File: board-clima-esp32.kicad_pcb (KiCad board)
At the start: 2 copper layers, 64.8 x 39.9 mm, 33 parts, among them IC1 ESP32-S3-WROOM-1-N4, J1 Conn_01x02_Pin, J2 Screw_Terminal_01x03, J3 Conn_01x04_Pin, J4 Conn_01x04_Pin, J5 Conn_01x04_Pin, J6 USB_C_Receptacle, Q1 AO3400A, SW1 RESET, SW2 BOOT, U1 AMS1117-3.3, U2 JZC-32F/C

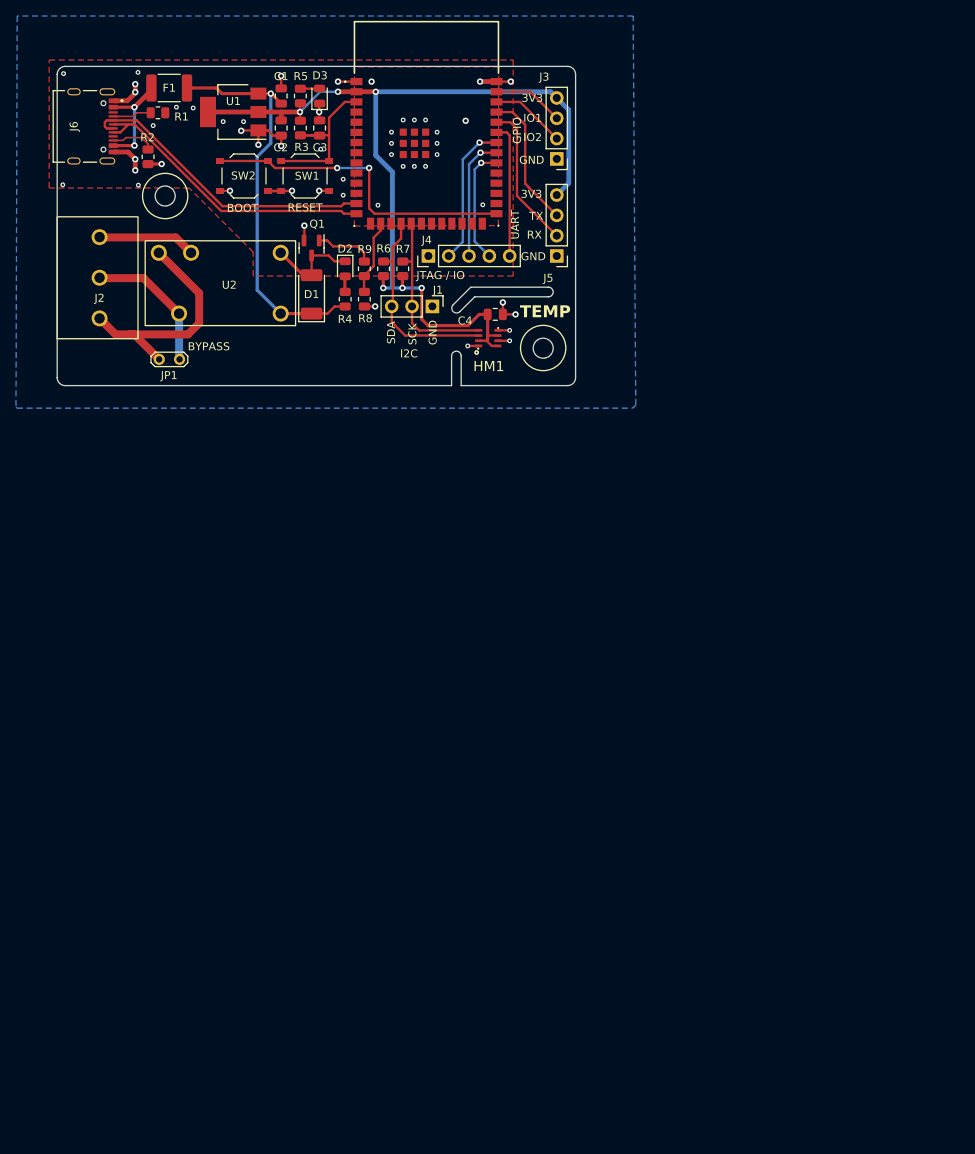
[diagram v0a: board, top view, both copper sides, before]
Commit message: pcb rev2 placement
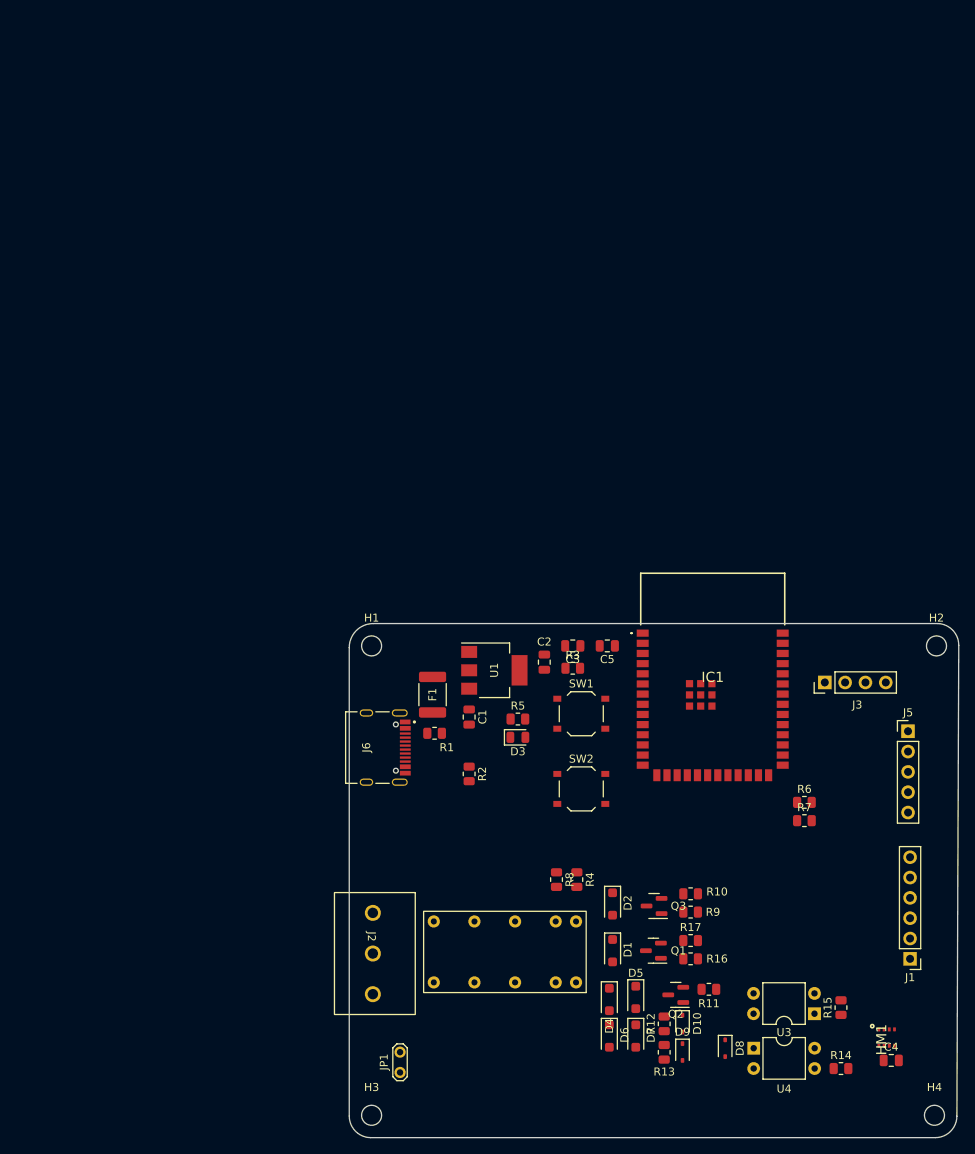
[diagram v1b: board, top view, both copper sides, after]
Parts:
- removed J4: Conn_01x04_Pin, Connector_PinHeader_2.54mm:PinHeader_1x05_P2.54mm_Vertical
- added C5: 1u, Capacitor_SMD:C_0805_2012Metric, F.Cu at (159.8, 126.2)
- added D10: 15V, Diode_SMD:D_SOD-323, F.Cu at (169.2, 173.4)
- added D4: SM4007PL, Diode_SMD:D_SOD-123F, F.Cu at (160.0, 170.4)
- added D5: SM4007PL, Diode_SMD:D_SOD-123F, F.Cu at (163.3, 170.2)
- added D6: SM4007PL, Diode_SMD:D_SOD-123F, F.Cu at (160.0, 175.0)
- added D7: SM4007PL, Diode_SMD:D_SOD-123F, F.Cu at (163.3, 175.0)
- added D8: 4V3, Diode_SMD:D_SOD-323, F.Cu at (174.5, 176.5)
- added D9: 4V7, Diode_SMD:D_SOD-323, F.Cu at (169.2, 177.0)
- added H3: MountingHole, MountingHole:MountingHole_2.5mm, F.Cu at (130.3, 184.9)
- added H4: MountingHole, MountingHole:MountingHole_2.5mm, F.Cu at (200.7, 184.9)
- added Q2: AO3401A, Package_TO_SOT_SMD:SOT-23, F.Cu at (168.3, 169.9)
- added Q3: AO3400A, Package_TO_SOT_SMD:SOT-23, F.Cu at (165.6, 158.8)
- added R10: 10k, Resistor_SMD:R_0805_2012Metric, F.Cu at (170.2, 157.2)
- added R11: 330, Resistor_SMD:R_0805_2012Metric, F.Cu at (172.5, 169.2)
- added R12: 220, Resistor_SMD:R_0805_2012Metric, F.Cu at (166.9, 173.5)
- added R13: 100, Resistor_SMD:R_0805_2012Metric, F.Cu at (166.9, 177.0)
- added R14: 10k, Resistor_SMD:R_0805_2012Metric, F.Cu at (189.0, 179.1)
- added R15: 330, Resistor_SMD:R_0805_2012Metric, F.Cu at (189.0, 171.4)
- added R16: 220, Resistor_SMD:R_0805_2012Metric, F.Cu at (170.2, 165.4)
- added R17: 10k, Resistor_SMD:R_0805_2012Metric, F.Cu at (170.2, 163.1)
- added U3: PC817, Package_DIP:DIP-4_W7.62mm, F.Cu at (185.7, 172.2)
- added U4: PC817, Package_DIP:DIP-4_W7.62mm, F.Cu at (178.1, 176.5)
- D1: value SM4007 -> SM4007PL; footprint Diode_SMD:D_MELF -> Diode_SMD:D_SOD-123F
- D2: value LED -> SM4007PL; footprint LED_SMD:LED_0805_2012Metric -> Diode_SMD:D_SOD-123F
- J1: value Conn_01x02_Pin -> Conn_01x06_Pin; footprint Connector_PinHeader_2.54mm:PinHeader_1x03_P2.54mm_Vertical -> Connector_PinHeader_2.54mm:PinHeader_1x06_P2.54mm_Vertical
- J5: value Conn_01x04_Pin -> Conn_01x05_Pin; footprint Connector_PinHeader_2.54mm:PinHeader_1x04_P2.54mm_Vertical -> Connector_PinHeader_2.54mm:PinHeader_1x05_P2.54mm_Vertical
- R4: value 220 -> 0
- R5: value 220 -> 1k
- R8: value 10k -> 0
- U2: value JZC-32F/C -> ~; footprint JZC-32FC:JZC-32FC -> HFD2:HFD2-00X-M-L2
- moved C4 105.6 mm to (195.3, 178.1)
- moved J1 101.1 mm to (197.6, 165.4), turned to 180 degrees
- moved HM1 99.7 mm to (193.7, 176.2), turned to 90 degrees
- moved Q1 97.7 mm to (165.5, 164.3), turned to 180 degrees
- moved JP1 93.3 mm to (133.9, 179.6), turned to 90 degrees
- moved U2 90.9 mm to (157.1, 169.6)
- moved D1 90.3 mm to (160.4, 164.3), turned to -90 degrees
- moved R9 90.2 mm to (170.2, 159.5), turned to 0 degrees
- moved SW2 87.4 mm to (156.5, 144.1)
- moved R2 87.0 mm to (142.5, 142.2)
- moved D2 86.1 mm to (160.4, 158.5)
- moved J6 85.8 mm to (129.7, 138.9)
- moved R7 85.3 mm to (184.4, 148.1), turned to 0 degrees
- moved R6 84.9 mm to (184.4, 145.8), turned to 0 degrees
- moved R1 84.9 mm to (138.2, 137.2)
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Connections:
- D1 pad 1: +5V -> Net-(D1-K)
- D2 pad 1: Net-(D1-A) -> Net-(D2-K)
- IC1 pad 16: /RELAY -> unconnected-(IC1-IO46-Pad16)
- IC1 pad 18: /SDA -> /BOILER_1
- IC1 pad 19: /SCK -> /BOILER_2
- IC1 pad 21: unconnected-(IC1-IO13-Pad21) -> /GPIO4
- IC1 pad 22: unconnected-(IC1-IO14-Pad22) -> /GPIO5
- IC1 pad 23: unconnected-(IC1-IO21-Pad23) -> /SDA
- IC1 pad 24: unconnected-(IC1-IO47-Pad24) -> /SCK
- IC1 pad 31: unconnected-(IC1-IO38-Pad31) -> /GPIO3
- IC1 pad 32: /JTAG_TCK -> unconnected-(IC1-IO39-Pad32)
- IC1 pad 33: /JTAG_TDO -> unconnected-(IC1-IO40-Pad33)
- IC1 pad 34: /JTAG_TDI -> unconnected-(IC1-IO41-Pad34)
- IC1 pad 35: /JTAG_TMS -> unconnected-(IC1-IO42-Pad35)
- IC1 pad 38: /GPIO2 -> /GPIO1
- IC1 pad 39: /GPIO1 -> /GPIO2
- J1 pad 1: GND -> /GPIO5
- J1 pad 2: /SCK -> /GPIO4
- J2 pad 3: Net-(J2-Pin_3) -> /R_NC
- J5 pad 1: GND -> /GPIO3
- J5 pad 4: +3.3V -> GND
- R4 pad 2: Net-(D2-A) -> Net-(D1-K)
- R6 pad 2: /SDA -> /SCK
- R7 pad 2: /SCK -> /SDA
- R8 pad 1: /RELAY -> +5V
- R8 pad 2: GND -> Net-(D2-K)
- R9 pad 1: /RELAY -> /BOILER_2
- R9 pad 2: Net-(Q1-G) -> Net-(Q3-G)
- U2 pad 1: +5V -> Net-(D1-A)
- U2 pad 2: Net-(D1-A) -> Net-(D2-A)
- U2 pad 4: Net-(J2-Pin_3) -> /R_COM
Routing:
- net +3.3V: track 114.0 -> 0.00 mm, vias 6 -> 0
- net +5V: track 50.4 -> 0.00 mm, vias 1 -> 0
- net GND: track 46.3 -> 0.00 mm, vias 51 -> 0
- net /BOOT: track 39.8 -> 0.00 mm, vias 2 -> 0
- net /USB-: track 37.4 -> 0.00 mm
- net /USB+: track 36.8 -> 0.00 mm
- net /R_NO: track 29.7 -> 0.00 mm
- net /SDA: track 25.1 -> 0.00 mm
- net /SCK: track 22.5 -> 0.00 mm
- net Net-(IC1-EN): track 21.2 -> 0.00 mm
- net /UART_RX: track 18.8 -> 0.00 mm
- net /JTAG_TDI: track 17.9 -> 0.00 mm, vias 1 -> 0
- net /UART_TX: track 17.6 -> 0.00 mm
- net /R_COM: track 17.5 -> 0.00 mm
- net /JTAG_TMS: track 17.3 -> 0.00 mm
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- removed copper zone on B.Cu, net GND
- removed copper zone on F.Cu, net GND
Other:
- board size 64.8 x 39.9 mm -> 76.2 x 64.3 mm
- board text removed: "${COMMENT1}"
- board text removed: "${COMPANY} ${REVISION} NO WARRANTY WHATSOEVER USAGE AT USER'S OWN RISK"
- board text removed: "3V3"
- board text removed: "BOOT"
- board text removed: "BYPASS"
- board text removed: "GND"
- board text removed: "GPIO"
- board text removed: "I2C"
- board text removed: "IO1"
- board text removed: "IO2"
- board text removed: "JTAG / IO"
- board text removed: "RESET"
- board text removed: "RX"
- board text removed: "SCK"
- board text removed: "SDA"
- board text removed: "TEMP"
- board text removed: "TX"
- board text removed: "UART"
